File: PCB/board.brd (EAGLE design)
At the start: 41 x 32 mm, 43 parts, among them J1 USB-A_PTH_MALE, U1 CH340E, U2 NRF52832, Y1 32MHz_2016, Y2 32.768kHz

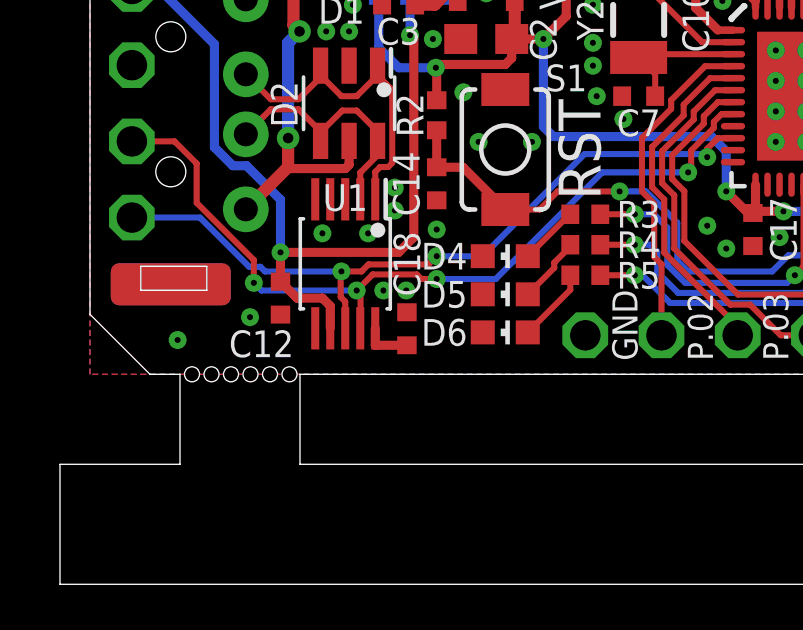
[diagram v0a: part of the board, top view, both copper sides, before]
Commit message: output files, dir cleanup
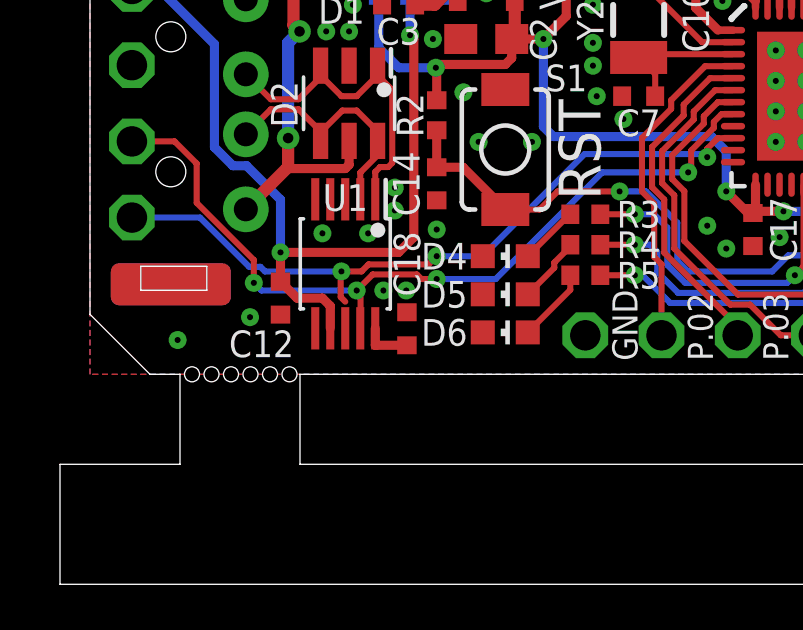
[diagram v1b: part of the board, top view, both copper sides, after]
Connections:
- net UART_RX: now also U1.9; no longer U1.8
- net UART_TX: now also U1.8; no longer U1.9
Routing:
- net UART_RX: track 24.8 -> 24.0 mm
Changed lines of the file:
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@@
 <layer number="25" name="tNames" color="7" fill="1" visible="yes" active="yes"/>
 <layer number="26" name="bNames" color="7" fill="1" visible="yes" active="yes"/>
-<layer number="27" name="tValues" color="7" fill="1" visible="yes" active="yes"/>
+<layer number="27" name="tValues" color="7" fill="1" visible="no" active="yes"/>
 <layer number="28" name="bValues" color="7" fill="1" visible="no" active="yes"/>
 <layer number="29" name="tStop" color="7" fill="3" visible="no" active="yes"/>
@@
 <via x="8.382" y="3.429" extent="1-16" drill="0.2"/>
 <contactref element="U2" pad="10"/>
-<contactref element="U1" pad="8"/>
-<wire x1="8.509" y1="1.533" x2="8.509" y2="2.42025625" width="0.2032" layer="1"/>
 <wire x1="8.509" y1="2.42025625" x2="8.35631875" y2="2.5729375" width="0.2032" layer="1"/>
 <wire x1="8.35631875" y1="3.40331875" x2="8.382" y2="3.429" width="0.2032" layer="1"/>
@@
 <wire x1="8.382" y1="3.429" x2="5.83474375" y2="3.429" width="0.2032" layer="16"/>
 <wire x1="5.30831875" y1="3.58168125" x2="3.666" y2="5.224" width="0.2032" layer="16"/>
+<contactref element="U1" pad="9"/>
+<wire x1="8.509" y1="2.42025625" x2="9.009" y2="1.533" width="0" layer="19" extent="1-1"/>
 </signal>
 <signal name="UART_TX">
@@
 <via x="8.89" y="2.794" extent="1-16" drill="0.2"/>
 <contactref element="U2" pad="8"/>
-<contactref element="U1" pad="9"/>
 <wire x1="9.017" y1="2.667" x2="9.017" y2="1.541" width="0.2032" layer="1"/>
-<wire x1="9.009" y1="1.533" x2="9.017" y2="1.541" width="0.2032" layer="1"/>
 <wire x1="8.89" y1="2.794" x2="9.017" y2="2.667" width="0.2032" layer="1"/>
 <wire x1="8.89" y1="2.794" x2="9.42368125" y2="3.32768125" width="0.2032" layer="1"/>
@@
 <wire x1="8.89" y1="2.794" x2="5.715" y2="2.794" width="0.2032" layer="16"/>
 <wire x1="3.556" y1="5.715" x2="3.556" y2="7.0261625" width="0.2032" layer="1"/>
+<contactref element="U1" pad="8"/>
+<wire x1="8.509" y1="1.533" x2="9.017" y2="1.541" width="0" layer="19" extent="1-1"/>
 </signal>
 <signal name="N$6">

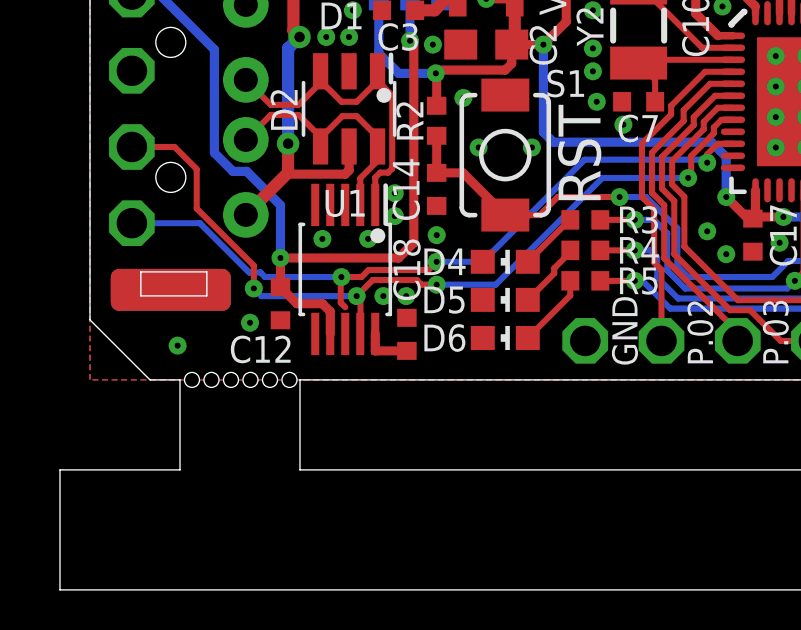
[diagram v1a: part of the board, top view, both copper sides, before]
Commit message: airwire error fix
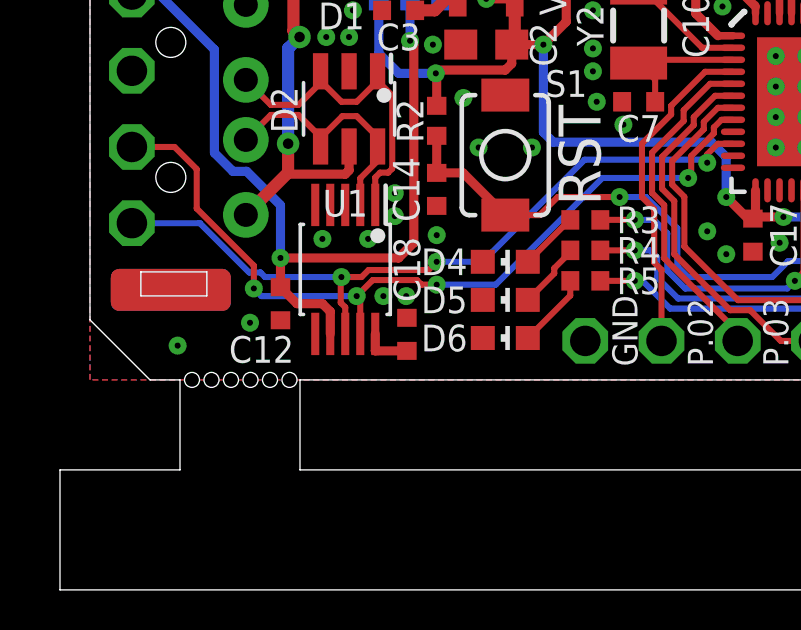
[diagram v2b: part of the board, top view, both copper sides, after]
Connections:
- net UART_RX: now also U1.8; no longer U1.9
- net UART_TX: now also U1.9; no longer U1.8
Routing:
- net UART_RX: track 24.0 -> 24.8 mm
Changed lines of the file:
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@@
 <setting verticaltext="up"/>
 </settings>
-<grid distance="5" unitdist="mil" unit="mil" style="lines" multiple="1" display="yes" altdistance="5" altunitdist="mil" altunit="mil"/>
+<grid distance="10" unitdist="mil" unit="mil" style="lines" multiple="1" display="yes" altdistance="5" altunitdist="mil" altunit="mil"/>
 <layers>
 <layer number="1" name="Top" color="4" fill="1" visible="yes" active="yes"/>
@@
 <via x="8.382" y="3.429" extent="1-16" drill="0.2"/>
 <contactref element="U2" pad="10"/>
-<wire x1="8.509" y1="2.42025625" x2="8.35631875" y2="2.5729375" width="0.2032" layer="1"/>
+<wire x1="8.35631875" y1="2.5729375" x2="8.509" y2="2.42025625" width="0.2032" layer="1"/>
 <wire x1="8.35631875" y1="3.40331875" x2="8.382" y2="3.429" width="0.2032" layer="1"/>
 <wire x1="8.35631875" y1="2.5729375" x2="8.35631875" y2="3.40331875" width="0.2032" layer="1"/>
@@
 <wire x1="8.382" y1="3.429" x2="5.83474375" y2="3.429" width="0.2032" layer="16"/>
 <wire x1="5.30831875" y1="3.58168125" x2="3.666" y2="5.224" width="0.2032" layer="16"/>
-<contactref element="U1" pad="9"/>
-<wire x1="8.509" y1="2.42025625" x2="9.009" y2="1.533" width="0" layer="19" extent="1-1"/>
+<contactref element="U1" pad="8"/>
+<wire x1="8.509" y1="2.42025625" x2="8.509" y2="1.533" width="0.2032" layer="1"/>
 </signal>
 <signal name="UART_TX">
@@
 <via x="8.89" y="2.794" extent="1-16" drill="0.2"/>
 <contactref element="U2" pad="8"/>
-<wire x1="9.017" y1="2.667" x2="9.017" y2="1.541" width="0.2032" layer="1"/>
 <wire x1="8.89" y1="2.794" x2="9.017" y2="2.667" width="0.2032" layer="1"/>
 <wire x1="8.89" y1="2.794" x2="9.42368125" y2="3.32768125" width="0.2032" layer="1"/>
@@
 <wire x1="8.89" y1="2.794" x2="5.715" y2="2.794" width="0.2032" layer="16"/>
 <wire x1="3.556" y1="5.715" x2="3.556" y2="7.0261625" width="0.2032" layer="1"/>
-<contactref element="U1" pad="8"/>
-<wire x1="8.509" y1="1.533" x2="9.017" y2="1.541" width="0" layer="19" extent="1-1"/>
+<contactref element="U1" pad="9"/>
+<wire x1="8.89" y1="2.794" x2="9.009" y2="2.675" width="0.2032" layer="1"/>
+<wire x1="9.009" y1="2.675" x2="9.009" y2="1.533" width="0.2032" layer="1"/>
 </signal>
 <signal name="N$6">
